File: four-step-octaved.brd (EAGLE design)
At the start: 100 x 80 mm, 36 parts, among them IC1 556, IC2 4017N, IC3 4040N, J1 BATTERY, J2 SPEAKER, U1 LM386N

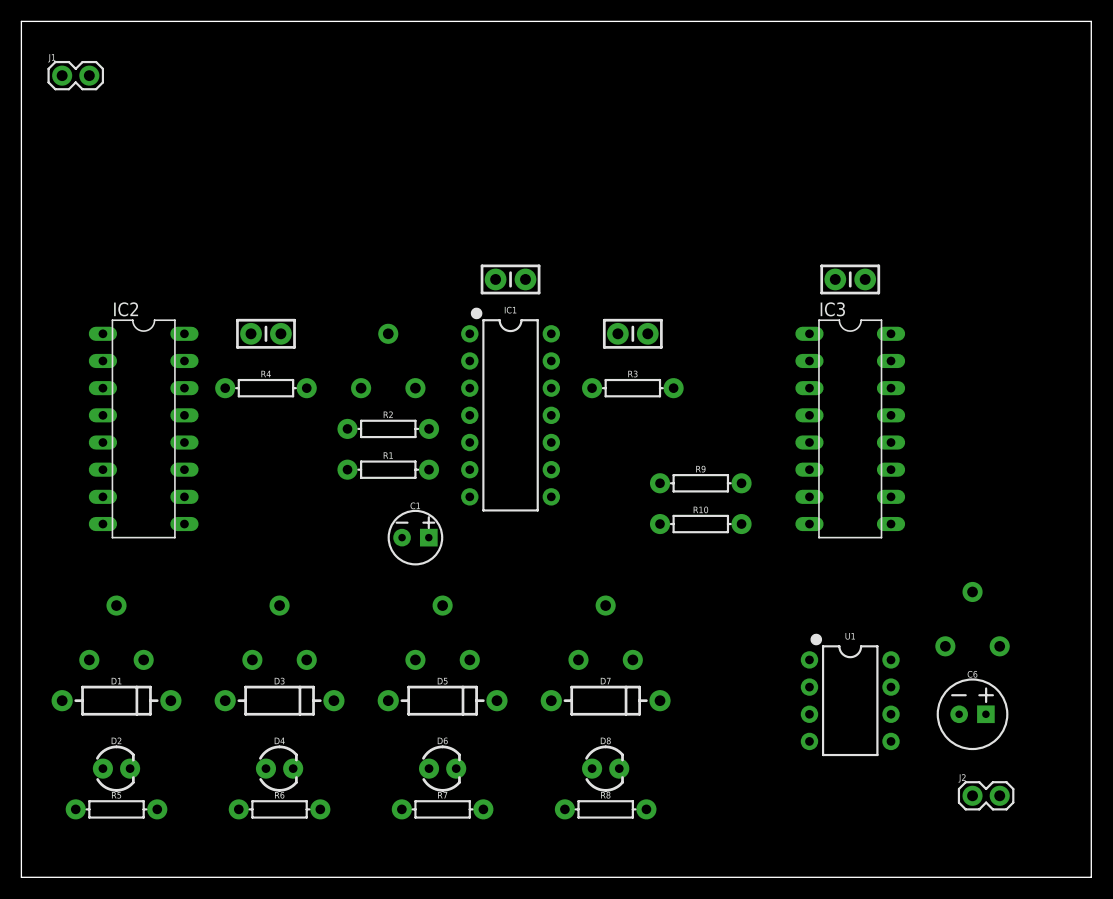
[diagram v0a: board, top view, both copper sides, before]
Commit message: Tidier board
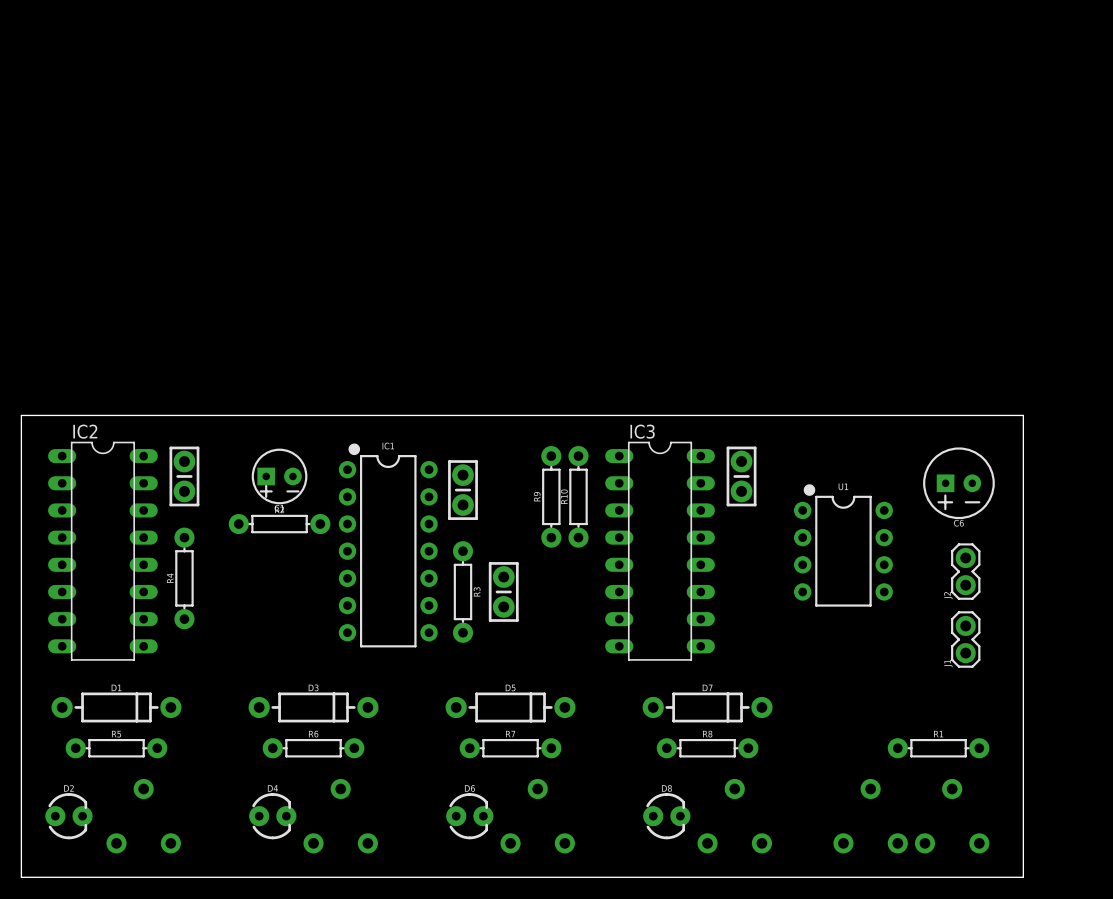
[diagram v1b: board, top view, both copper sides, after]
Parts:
- moved J1 100.2 mm to (88.3, 21.0), turned to 90 degrees
- moved RV1 67.7 mm to (87.0, 3.17)
- moved R1 57.6 mm to (85.7, 12.1)
- moved C3 27.0 mm to (45.1, 26.7), turned to 270 degrees
- moved R3 24.8 mm to (41.3, 26.7), turned to 270 degrees
- moved C6 21.6 mm to (87.6, 36.8), turned to 180 degrees
- moved IC3 21.1 mm to (59.7, 30.5)
- moved C5 21.0 mm to (67.3, 37.5), turned to 270 degrees
- moved RV5 21.0 mm to (66.7, 3.17)
- moved RV6 20.7 mm to (79.4, 3.17)
- moved C2 20.2 mm to (41.3, 36.2), turned to 270 degrees
- moved J2 19.7 mm to (88.3, 27.3), turned to 90 degrees
- moved R4 19.3 mm to (15.2, 27.9), turned to 90 degrees
- moved RV4 19.3 mm to (48.3, 3.17)
- moved RV3 18.1 mm to (29.8, 3.17)
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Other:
- board size 100 x 80 mm -> 93.7 x 43.2 mm
